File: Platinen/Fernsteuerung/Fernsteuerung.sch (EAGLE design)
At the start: 2 parts, among them K1 ESP32DEVKITV11000MIL, P1 TFT_3.5"_SPI_480X320

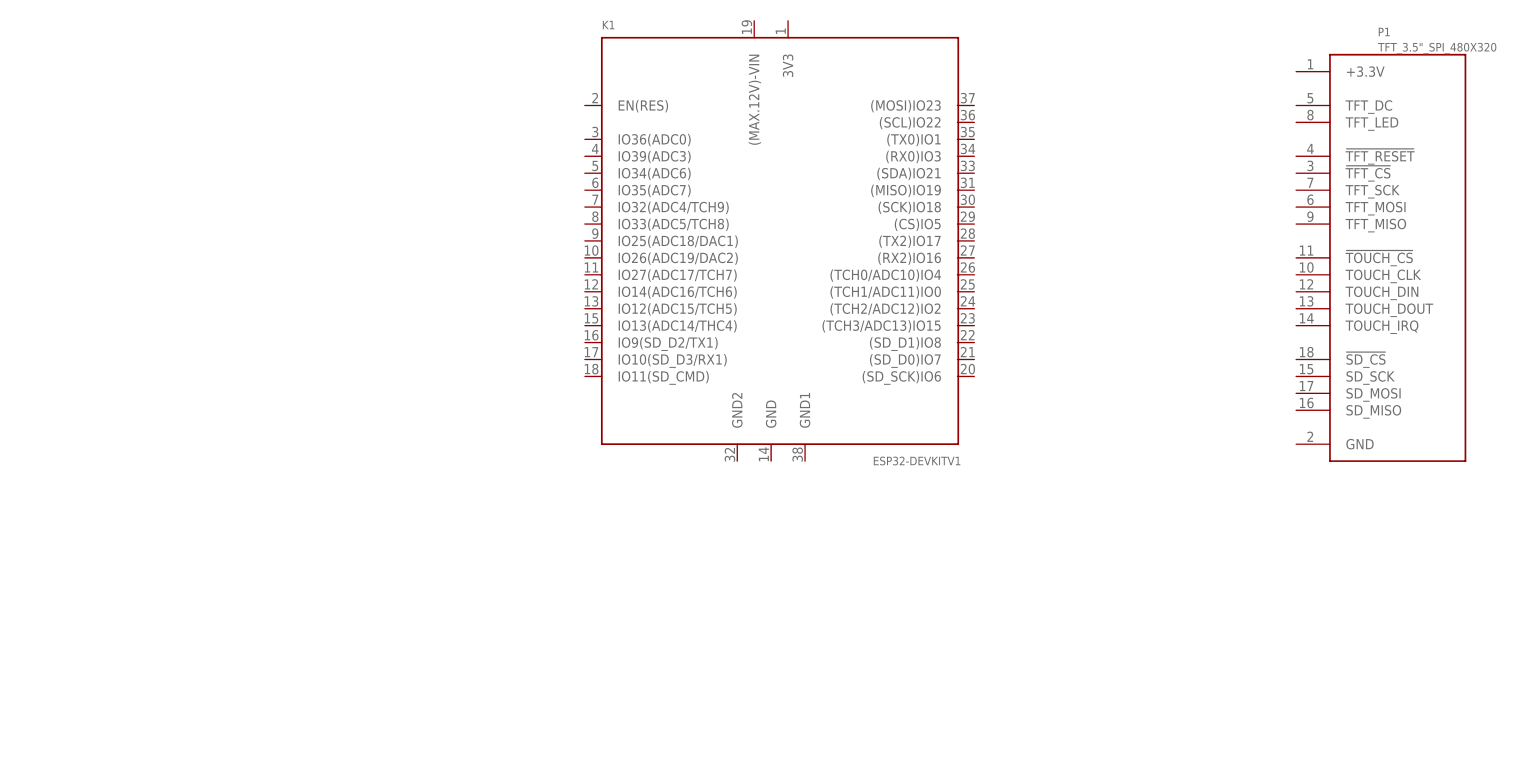
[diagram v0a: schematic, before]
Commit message: Freitag commit
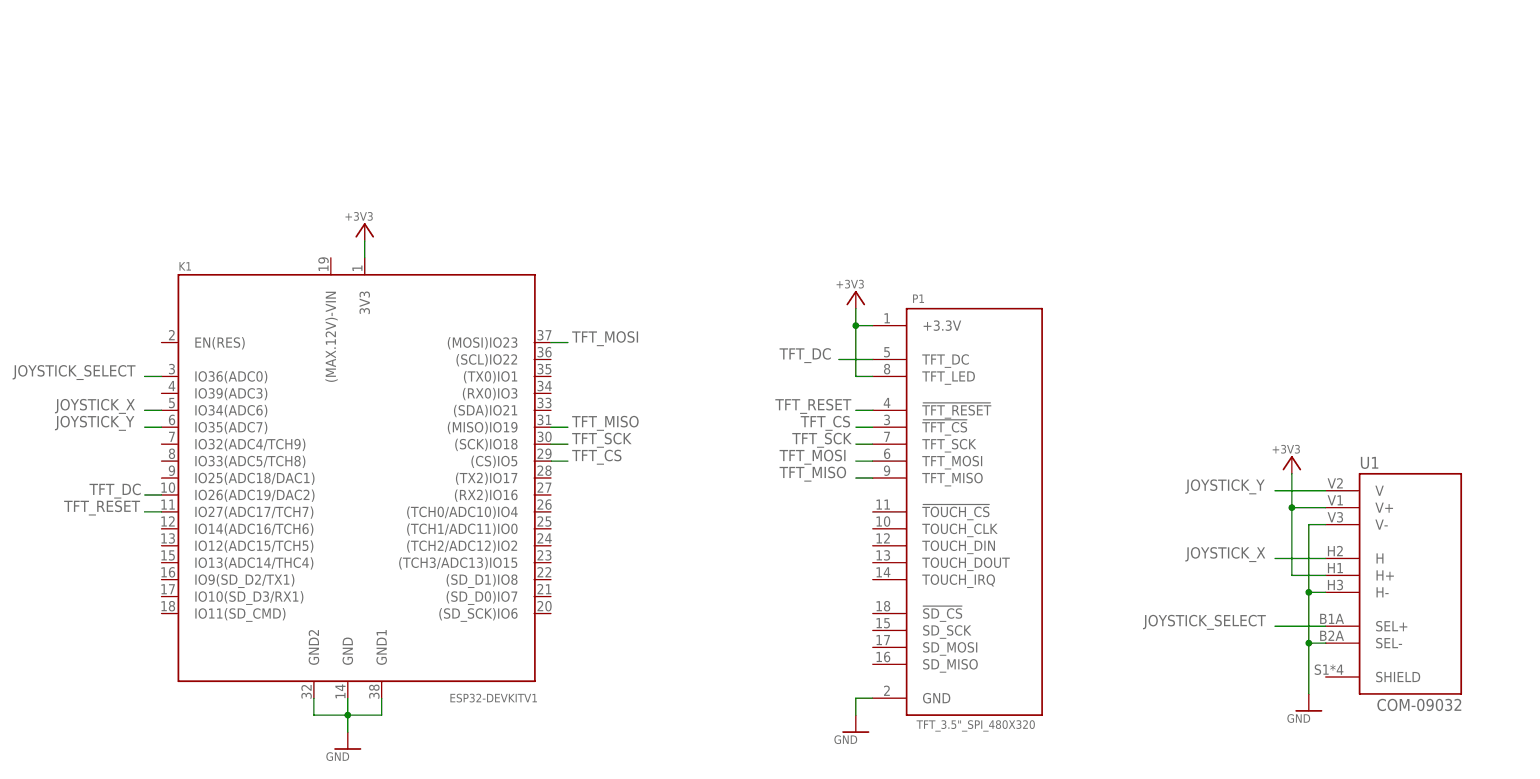
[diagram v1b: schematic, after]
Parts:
- added U1: COM-09032, joystick COM-09032:COM-09032
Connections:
- new net +3V3: K1.3V3, P1.+3.3V, P1.TFT_LED, U1.H+, U1.V+
- new net GND: K1.GND, K1.GND1, K1.GND2, P1.GND, U1.H-, U1.SEL-, U1.V-
- new net JOYSTICK_SELECT: K1.IO36(ADC0), U1.SEL+
- new net JOYSTICK_X: K1.IO34(ADC6), U1.H
- new net JOYSTICK_Y: K1.IO35(ADC7), U1.V
- new net TFT_CS: K1.(CS)IO5, P1.!TFT_CS!
- new net TFT_DC: K1.IO26(ADC19/DAC2), P1.TFT_DC
- new net TFT_MISO: K1.(MISO)IO19, P1.TFT_MISO
- new net TFT_MOSI: K1.(MOSI)IO23, P1.TFT_MOSI
- new net TFT_RESET: K1.IO27(ADC17/TCH7), P1.!TFT_RESET!
- new net TFT_SCK: K1.(SCK)IO18, P1.TFT_SCK
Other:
- moved on the sheet: K1, P1
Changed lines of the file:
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@@
 <part name="K1" library="HTL22_Eagle7_Controller" deviceset="ESP32DEVKITV1" device="1000MIL"/>
 <part name="P1" library="TFT SPI 3.5inch 480x320 ILI9488" deviceset="TFT_3.5&quot;_SPI_480X320" device=""/>
+<part name="U1" library="joystick COM-09032" deviceset="COM-09032" device=""/>
+<part name="GND1" library="HTL22_basis" deviceset="GND" device=""/>
+<part name="+3V1" library="HTL22_basis" deviceset="+3V3" device=""/>
+<part name="GND2" library="HTL22_basis" deviceset="GND" device=""/>
+<part name="+3V2" library="HTL22_basis" deviceset="+3V3" device=""/>
+<part name="+3V3" library="HTL22_basis" deviceset="+3V3" device=""/>
+<part name="GND3" library="HTL22_basis" deviceset="GND" device=""/>
 </parts>
 <sheets>
@@
 </plain>
 <instances>
-<instance part="K1" gate="G$1" x="119.38" y="78.74"/>
-<instance part="P1" gate="G$1" x="213.36" y="76.2"/>
+<instance part="K1" gate="G$1" x="55.88" y="43.18" smashed="yes">
+<attribute name="NAME" x="30.48" y="74.295" size="1.27" layer="95"/>
+</instance>
+<instance part="P1" gate="G$1" x="149.86" y="38.1" smashed="yes">
+<attribute name="NAME" x="140.5128" y="69.4436" size="1.27" layer="95" ratio="12"/>
+<attribute name="VALUE" x="141.1986" y="5.5626" size="1.27" layer="96" ratio="12"/>
+</instance>
+<instance part="U1" gate="G$1" x="215.265" y="28.575" smashed="yes">
+<attribute name="NAME" x="207.645" y="44.577" size="1.778" layer="95"/>
+<attribute name="VALUE" x="210.185" y="8.255" size="1.778" layer="96"/>
+</instance>
+<instance part="GND1" gate="1" x="200.025" y="8.255"/>
+<instance part="+3V1" gate="G$1" x="197.485" y="46.355"/>
+<instance part="GND2" gate="1" x="55.88" y="2.54"/>
+<instance part="+3V2" gate="G$1" x="58.42" y="81.28"/>
+<instance part="+3V3" gate="G$1" x="132.08" y="71.12"/>
+<instance part="GND3" gate="1" x="132.08" y="5.08"/>
 </instances>
 <busses>
 </busses>
 <nets>
+<net name="+3V3" class="0">
+<segment>
+<pinref part="U1" gate="G$1" pin="V+"/>
+<wire x1="202.565" y1="38.735" x2="197.485" y2="38.735" width="0.1524" layer="91"/>
+<wire x1="197.485" y1="38.735" x2="197.485" y2="28.575" width="0.1524" layer="91"/>
+<pinref part="U1" gate="G$1" pin="H+"/>
+<wire x1="197.485" y1="28.575" x2="202.565" y2="28.575" width="0.1524" layer="91"/>
+<wire x1="197.485" y1="38.735" x2="197.485" y2="43.815" width="0.1524" layer="91"/>
+<junction x="197.485" y="38.735"/>
+<pinref part="+3V1" gate="G$1" pin="+3V3"/>
+</segment>
+<segment>
+<pinref part="K1" gate="G$1" pin="3V3"/>
+<wire x1="58.42" y1="76.2" x2="58.42" y2="78.74" width="0.1524" layer="91"/>
+<pinref part="+3V2" gate="G$1" pin="+3V3"/>
+</segment>
+<segment>
+<wire x1="132.08" y1="68.58" x2="132.08" y2="66.04" width="0.1524" layer="91"/>
+<pinref part="P1" gate="G$1" pin="+3.3V"/>
+<wire x1="132.08" y1="66.04" x2="134.62" y2="66.04" width="0.1524" layer="91"/>
+<pinref part="+3V3" gate="G$1" pin="+3V3"/>
+<pinref part="P1" gate="G$1" pin="TFT_LED"/>
+<wire x1="134.62" y1="58.42" x2="132.08" y2="58.42" width="0.1524" layer="91"/>
+<wire x1="132.08" y1="58.42" x2="132.08" y2="66.04" width="0.1524" layer="91"/>
+<junction x="132.08" y="66.04"/>
+</segment>
+</net>
+<net name="GND" class="0">
+<segment>
+<pinref part="U1" gate="G$1" pin="V-"/>
+<wire x1="202.565" y1="36.195" x2="200.025" y2="36.195" width="0.1524" layer="91"/>
+<wire x1="200.025" y1="36.195" x2="200.025" y2="26.035" width="0.1524" layer="91"/>
+<pinref part="U1" gate="G$1" pin="H-"/>
+<wire x1="200.025" y1="26.035" x2="202.565" y2="26.035" width="0.1524" layer="91"/>
+<wire x1="200.025" y1="26.035" x2="200.025" y2="18.415" width="0.1524" layer="91"/>
+<junction x="200.025" y="26.035"/>
+<pinref part="U1" gate="G$1" pin="SEL-"/>
+<wire x1="200.025" y1="18.415" x2="202.565" y2="18.415" width="0.1524" layer="91"/>
+<wire x1="200.025" y1="18.415" x2="200.025" y2="10.795" width="0.1524" layer="91"/>
+<junction x="200.025" y="18.415"/>
+<pinref part="GND1" gate="1" pin="GND"/>
+</segment>
+<segment>
+<pinref part="GND2" gate="1" pin="GND"/>
+<pinref part="K1" gate="G$1" pin="GND"/>
+<wire x1="55.88" y1="5.08" x2="55.88" y2="7.62" width="0.1524" layer="91"/>
+<pinref part="K1" gate="G$1" pin="GND1"/>
+<wire x1="55.88" y1="7.62" x2="55.88" y2="10.16" width="0.1524" layer="91"/>
+<wire x1="55.88" y1="7.62" x2="60.96" y2="7.62" width="0.1524" layer="91"/>
+<wire x1="60.96" y1="7.62" x2="60.96" y2="10.16" width="0.1524" layer="91"/>
+<junction x="55.88" y="7.62"/>
+<pinref part="K1" gate="G$1" pin="GND2"/>
+<wire x1="55.88" y1="7.62" x2="50.8" y2="7.62" width="0.1524" layer="91"/>
+<wire x1="50.8" y1="7.62" x2="50.8" y2="10.16" width="0.1524" layer="91"/>
+</segment>
+<segment>
+<pinref part="P1" gate="G$1" pin="GND"/>
+<pinref part="GND3" gate="1" pin="GND"/>
+<wire x1="134.62" y1="10.16" x2="132.08" y2="10.16" width="0.1524" layer="91"/>
+<wire x1="132.08" y1="10.16" x2="132.08" y2="7.62" width="0.1524" layer="91"/>
+</segment>
+</net>
+<net name="JOYSTICK_SELECT" class="0">
+<segment>
+<pinref part="U1" gate="G$1" pin="SEL+"/>
+<wire x1="202.565" y1="20.955" x2="194.945" y2="20.955" width="0.1524" layer="91"/>
+<label x="175.26" y="20.955" size="1.6764" layer="95"/>
+</segment>
+<segment>
+<pinref part="K1" gate="G$1" pin="IO36(ADC0)"/>
+<wire x1="25.4" y1="58.42" x2="27.94" y2="58.42" width="0.1524" layer="91"/>
+<label x="5.715" y="58.42" size="1.6764" layer="95"/>
+</segment>
+</net>
+<net name="TFT_MOSI" class="0">
+<segment>
+<pinref part="K1" gate="G$1" pin="(MOSI)IO23"/>
+<wire x1="86.36" y1="63.5" x2="88.9" y2="63.5" width="0.1524" layer="91"/>
+<label x="89.535" y="63.5" size="1.6764" layer="95"/>
+</segment>
+<segment>
+<pinref part="P1" gate="G$1" pin="TFT_MOSI"/>
+<wire x1="134.62" y1="45.72" x2="132.08" y2="45.72" width="0.1524" layer="91"/>
+<label x="120.65" y="45.72" size="1.6764" layer="95"/>
+</segment>
+</net>
+<net name="TFT_MISO" class="0">
+<segment>
+<pinref part="K1" gate="G$1" pin="(MISO)IO19"/>
+<wire x1="86.36" y1="50.8" x2="88.9" y2="50.8" width="0.1524" layer="91"/>
+<label x="89.535" y="50.8" size="1.6764" layer="95"/>
+</segment>
+<segment>
+<pinref part="P1" gate="G$1" pin="TFT_MISO"/>
+<wire x1="134.62" y1="43.18" x2="132.08" y2="43.18" width="0.1524" layer="91"/>
+<label x="120.65" y="43.18" size="1.6764" layer="95"/>
+</segment>
+</net>
+<net name="TFT_SCK" class="0">
+<segment>
+<pinref part="K1" gate="G$1" pin="(SCK)IO18"/>
+<wire x1="86.36" y1="48.26" x2="88.9" y2="48.26" width="0.1524" layer="91"/>
+<label x="89.535" y="48.26" size="1.6764" layer="95"/>
+</segment>
+<segment>
+<pinref part="P1" gate="G$1" pin="TFT_SCK"/>
+<wire x1="134.62" y1="48.26" x2="132.08" y2="48.26" width="0.1524" layer="91"/>
+<label x="122.555" y="48.26" size="1.6764" layer="95"/>
+</segment>
+</net>
+<net name="TFT_CS" class="0">
+<segment>
+<pinref part="K1" gate="G$1" pin="(CS)IO5"/>
+<wire x1="86.36" y1="45.72" x2="88.9" y2="45.72" width="0.1524" layer="91"/>
+<label x="89.535" y="45.72" size="1.6764" layer="95"/>
+</segment>
+<segment>
+<pinref part="P1" gate="G$1" pin="!TFT_CS!"/>
+<wire x1="134.62" y1="50.8" x2="132.08" y2="50.8" width="0.1524" layer="91"/>
+<label x="123.825" y="50.8" size="1.6764" layer="95"/>
+</segment>
+</net>
+<net name="TFT_DC" class="0">
+<segment>
+<pinref part="K1" gate="G$1" pin="IO26(ADC19/DAC2)"/>
+<wire x1="27.94" y1="40.64" x2="25.4" y2="40.64" width="0.1524" layer="91"/>
+<label x="17.145" y="40.64" size="1.6764" layer="95"/>
+</segment>
+<segment>
+<pinref part="P1" gate="G$1" pin="TFT_DC"/>
+<wire x1="134.62" y1="60.96" x2="129.54" y2="60.96" width="0.1524" layer="91"/>
+<label x="120.65" y="60.96" size="1.6764" layer="95"/>
+</segment>
+</net>
+<net name="TFT_RESET" class="0">
+<segment>
+<pinref part="K1" gate="G$1" pin="IO27(ADC17/TCH7)"/>
+<wire x1="27.94" y1="38.1" x2="25.4" y2="38.1" width="0.1524" layer="91"/>
+<label x="13.335" y="38.1" size="1.6764" layer="95"/>
+</segment>
+<segment>
+<pinref part="P1" gate="G$1" pin="!TFT_RESET!"/>
+<wire x1="134.62" y1="53.34" x2="132.08" y2="53.34" width="0.1524" layer="91"/>
+<label x="120.015" y="53.34" size="1.6764" layer="95"/>
+</segment>
+</net>
+<net name="JOYSTICK_X" class="0">
+<segment>
+<pinref part="U1" gate="G$1" pin="H"/>
+<wire x1="202.565" y1="31.115" x2="194.945" y2="31.115" width="0.1524" layer="91"/>
+<label x="181.61" y="31.115" size="1.6764" layer="95"/>
+</segment>
+<segment>
+<pinref part="K1" gate="G$1" pin="IO34(ADC6)"/>
+<wire x1="27.94" y1="53.34" x2="25.4" y2="53.34" width="0.1524" layer="91"/>
+<label x="12.065" y="53.34" size="1.6764" layer="95"/>
+</segment>
+</net>
+<net name="JOYSTICK_Y" class="0">
+<segment>
+<pinref part="U1" gate="G$1" pin="V"/>
+<wire x1="202.565" y1="41.275" x2="194.945" y2="41.275" width="0.1524" layer="91"/>
+<label x="181.61" y="41.275" size="1.6764" layer="95"/>
+</segment>
+<segment>
+<pinref part="K1" gate="G$1" pin="IO35(ADC7)"/>
+<wire x1="27.94" y1="50.8" x2="25.4" y2="50.8" width="0.1524" layer="91"/>
+<label x="12.065" y="50.8" size="1.6764" layer="95"/>
+</segment>
+</net>
 </nets>
 </sheet>
